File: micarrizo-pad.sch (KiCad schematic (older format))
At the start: 17 parts

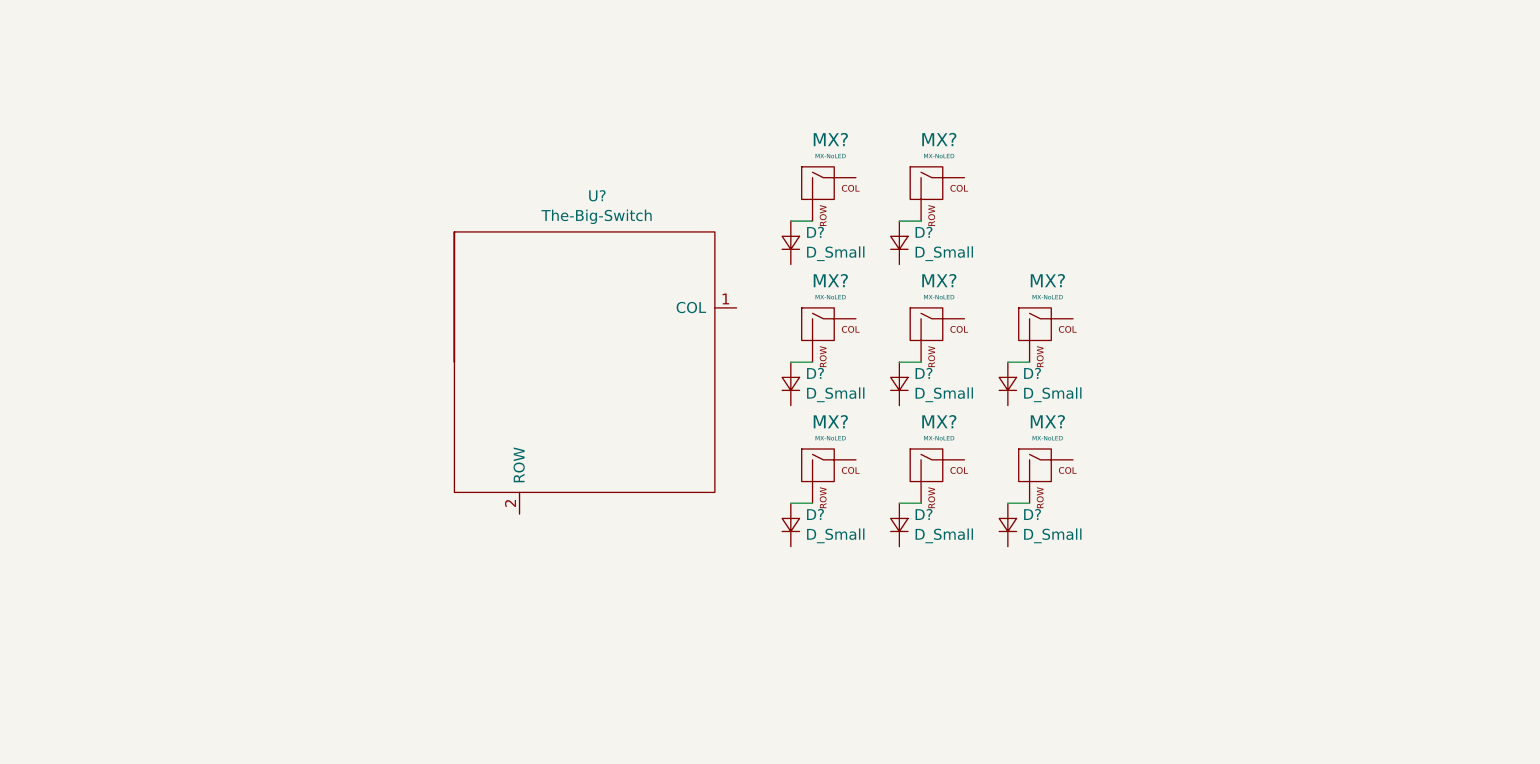
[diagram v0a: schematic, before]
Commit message: add rows cols
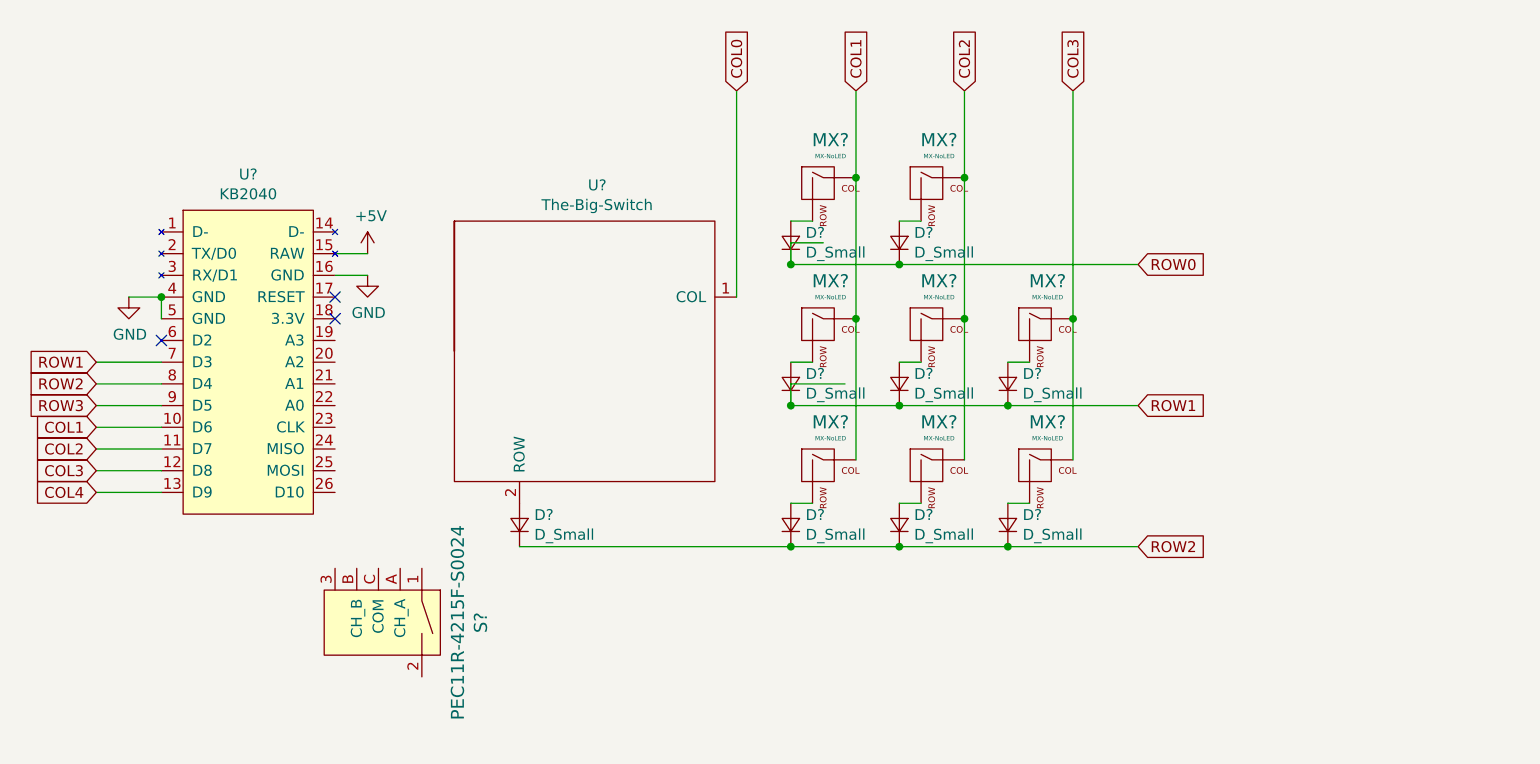
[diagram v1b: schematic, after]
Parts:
- added D?: D_Small, symbol Device:D_Small
- added S?: PEC11R-4215F-S0024, digikey-footprints:Rotary_Encoder_Switched_PEC11R, symbol dk_Encoders:PEC11R-4215F-S0024
- added U?: KB2040, symbol New_Library:KB2040
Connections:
- net labels added: +5V, COL0, COL1, COL2, COL3, COL4, GND, ROW0, ROW1, ROW2, ROW3
- wire segments 8 -> 41
- no-connect marks 0 -> 3
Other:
- moved on the sheet: U?
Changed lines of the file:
@@
 	5750 4300 5850 4300
+$Comp
+L Device:D_Small D?
+U 1 1 65EF06FC
+P 6250 4400
+F 0 "D?" V 6296 4332 50  0000 R CNN
+F 1 "D_Small" V 6205 4332 50  0000 R CNN
+F 2 "" V 6250 4400 50  0001 C CNN
+F 3 "~" V 6250 4400 50  0001 C CNN
+	1    6250 4400
+	0    -1   -1   0
+$EndComp
+Wire Wire Line
+	6250 4300 6350 4300
+$Comp
+L MX_Alps_Hybrid:MX-NoLED MX?
+U 1 1 65EF11E9
+P 6900 4150
+F 0 "MX?" H 6933 4373 60  0000 C CNN
+F 1 "MX-NoLED" H 6933 4299 20  0000 C CNN
+F 2 "" H 6275 4125 60  0001 C CNN
+F 3 "" H 6275 4125 60  0001 C CNN
+	1    6900 4150
+	1    0    0    -1
+$EndComp
+$Comp
+L Device:D_Small D?
+U 1 1 65EF11EF
+P 6750 4400
+F 0 "D?" V 6796 4332 50  0000 R CNN
+F 1 "D_Small" V 6705 4332 50  0000 R CNN
+F 2 "" V 6750 4400 50  0001 C CNN
+F 3 "~" V 6750 4400 50  0001 C CNN
+	1    6750 4400
+	0    -1   -1   0
+$EndComp
+Wire Wire Line
+	6750 4300 6850 4300
+$Comp
+L MX_Alps_Hybrid:MX-NoLED MX?
+U 1 1 65F09C65
+P 5900 2850
+F 0 "MX?" H 5933 3073 60  0000 C CNN
+F 1 "MX-NoLED" H 5933 2999 20  0000 C CNN
+F 2 "" H 5275 2825 60  0001 C CNN
+F 3 "" H 5275 2825 60  0001 C CNN
+	1    5900 2850
+	1    0    0    -1
+$EndComp
+$Comp
+L Device:D_Small D?
+U 1 1 65F09C6B
+P 5750 3100
+F 0 "D?" V 5796 3032 50  0000 R CNN
+F 1 "D_Small" V 5705 3032 50  0000 R CNN
+F 2 "" V 5750 3100 50  0001 C CNN
+F 3 "~" V 5750 3100 50  0001 C CNN
+	1    5750 3100
+	0    -1   -1   0
+$EndComp
+Wire Wire Line
+	5750 3000 5850 3000
+$Comp
+L MX_Alps_Hybrid:MX-NoLED MX?
+U 1 1 65F09C72
+P 6400 2850
+F 0 "MX?" H 6433 3073 60  0000 C CNN
+F 1 "MX-NoLED" H 6433 2999 20  0000 C CNN
+F 2 "" H 5775 2825 60  0001 C CNN
+F 3 "" H 5775 2825 60  0001 C CNN
+	1    6400 2850
+	1    0    0    -1
+$EndComp
+$Comp
+L Device:D_Small D?
+U 1 1 65F09C78
+P 6250 3100
+F 0 "D?" V 6296 3032 50  0000 R CNN
+F 1 "D_Small" V 6205 3032 50  0000 R CNN
+F 2 "" V 6250 3100 50  0001 C CNN
+F 3 "~" V 6250 3100 50  0001 C CNN
+	1    6250 3100
+	0    -1   -1   0
+$EndComp
+Wire Wire Line
+	6250 3000 6350 3000
+$Comp
+L New_Library:The-Big-Switch U?
+U 1 1 65F2656C
+P 4800 3600
+F 0 "U?" H 4858 4365 50  0000 C CNN
+F 1 "The-Big-Switch" H 4858 4274 50  0000 C CNN
+F 2 "" H 4250 4250 50  0001 C CNN
+F 3 "" H 4250 4250 50  0001 C CNN
+	1    4800 3600
+	1    0    0    -1
+$EndComp
+$Comp
+L New_Library:KB2040 U?
+U 1 1 65F497B3
+P 3250 3650
+F 0 "U?" H 3250 4515 50  0000 C CNN
+F 1 "KB2040" H 3250 4424 50  0000 C CNN
+F 2 "" H 3400 4400 50  0001 C CNN
+F 3 "" H 3400 4400 50  0001 C CNN
+	1    3250 3650
+	1    0    0    -1
+$EndComp
+$Comp
+L Device:D_Small D?
+U 1 1 65F4CF1E
+P 4500 4400
+F 0 "D?" V 4546 4332 50  0000 R CNN
+F 1 "D_Small" V 4455 4332 50  0000 R CNN
+F 2 "" V 4500 4400 50  0001 C CNN
+F 3 "~" V 4500 4400 50  0001 C CNN
+	1    4500 4400
+	0    -1   -1   0
+$EndComp
+Wire Wire Line
+	2850 3350 2850 3450
+Wire Wire Line
+	2700 3350 2850 3350
+Connection ~ 2850 3350
+$Comp
+L power:GND #PWR?
+U 1 1 65F4F1ED
+P 2700 3350
+F 0 "#PWR?" H 2700 3100 50  0001 C CNN
+F 1 "GND" H 2705 3177 50  0000 C CNN
+F 2 "" H 2700 3350 50  0001 C CNN
+F 3 "" H 2700 3350 50  0001 C CNN
+	1    2700 3350
+	1    0    0    -1
+$EndComp
+Wire Wire Line
+	3650 3250 3800 3250
+$Comp
+L power:GND #PWR?
+U 1 1 65F51406
+P 3800 3250
+F 0 "#PWR?" H 3800 3000 50  0001 C CNN
+F 1 "GND" H 3805 3077 50  0000 C CNN
+F 2 "" H 3800 3250 50  0001 C CNN
+F 3 "" H 3800 3250 50  0001 C CNN
+	1    3800 3250
+	1    0    0    -1
+$EndComp
+Wire Wire Line
+	3650 3150 3800 3150
+$Comp
+L power:+5V #PWR?
+U 1 1 65F51F24
+P 3800 3150
+F 0 "#PWR?" H 3800 3000 50  0001 C CNN
+F 1 "+5V" H 3815 3323 50  0000 C CNN
+F 2 "" H 3800 3150 50  0001 C CNN
+F 3 "" H 3800 3150 50  0001 C CNN
+	1    3800 3150
+	1    0    0    -1
+$EndComp
+Wire Wire Line
+	4500 4500 5750 4500
+Connection ~ 5750 4500
+Wire Wire Line
+	5750 4500 6250 4500
+Connection ~ 6250 4500
+Wire Wire Line
+	6250 4500 6750 4500
+Connection ~ 6750 4500
+Wire Wire Line
+	6750 4500 7350 4500
+Text GLabel 7350 3850 2    50   Input ~ 0
+ROW1
+Wire Wire Line
+	6000 3750 5750 3750
+Wire Wire Line
+	5750 3750 5750 3850
+Wire Wire Line
+	5750 3850 6250 3850
+Connection ~ 5750 3850
+Connection ~ 6250 3850
+Wire Wire Line
+	6250 3850 6750 3850
+Connection ~ 6750 3850
+Wire Wire Line
+	6750 3850 7350 3850
+Text GLabel 7350 4500 2    50   Input ~ 0
+ROW2
+Wire Wire Line
+	5900 3100 5750 3100
+Wire Wire Line
+	5750 3100 5750 3200
+Wire Wire Line
+	5750 3200 6250 3200
+Connection ~ 5750 3200
+Connection ~ 6250 3200
+Wire Wire Line
+	6250 3200 7350 3200
+Text GLabel 7350 3200 2    50   Input ~ 0
+ROW0
+Wire Wire Line
+	5500 3350 5500 2400
+Text GLabel 6050 2400 1    50   Input ~ 0
+COL1
+Wire Wire Line
+	6050 4100 6050 3450
+Connection ~ 6050 2800
+Wire Wire Line
+	6050 2800 6050 2400
+Connection ~ 6050 3450
+Wire Wire Line
+	6050 3450 6050 2800
+Text GLabel 6550 2400 1    50   Input ~ 0
+COL2
 $Comp
 L MX_Alps_Hybrid:MX-NoLED MX?
@@
 	1    0    0    -1
 $EndComp
-$Comp
-L Device:D_Small D?
-U 1 1 65EF06FC
-P 6250 4400
-F 0 "D?" V 6296 4332 50  0000 R CNN
-F 1 "D_Small" V 6205 4332 50  0000 R CNN
-F 2 "" V 6250 4400 50  0001 C CNN
-F 3 "~" V 6250 4400 50  0001 C CNN
-	1    6250 4400
-	0    -1   -1   0
-$EndComp
-Wire Wire Line
-	6250 4300 6350 4300
-$Comp
-L MX_Alps_Hybrid:MX-NoLED MX?
-U 1 1 65EF11E9
-P 6900 4150
-F 0 "MX?" H 6933 4373 60  0000 C CNN
-F 1 "MX-NoLED" H 6933 4299 20  0000 C CNN
-F 2 "" H 6275 4125 60  0001 C CNN
-F 3 "" H 6275 4125 60  0001 C CNN
-	1    6900 4150
-	1    0    0    -1
-$EndComp
-$Comp
-L Device:D_Small D?
-U 1 1 65EF11EF
-P 6750 4400
-F 0 "D?" V 6796 4332 50  0000 R CNN
-F 1 "D_Small" V 6705 4332 50  0000 R CNN
-F 2 "" V 6750 4400 50  0001 C CNN
-F 3 "~" V 6750 4400 50  0001 C CNN
-	1    6750 4400
-	0    -1   -1   0
-$EndComp
-Wire Wire Line
-	6750 4300 6850 4300
-$Comp
-L MX_Alps_Hybrid:MX-NoLED MX?
-U 1 1 65F09C65
-P 5900 2850
-F 0 "MX?" H 5933 3073 60  0000 C CNN
-F 1 "MX-NoLED" H 5933 2999 20  0000 C CNN
-F 2 "" H 5275 2825 60  0001 C CNN
-F 3 "" H 5275 2825 60  0001 C CNN
-	1    5900 2850
-	1    0    0    -1
-$EndComp
-$Comp
-L Device:D_Small D?
-U 1 1 65F09C6B
-P 5750 3100
-F 0 "D?" V 5796 3032 50  0000 R CNN
-F 1 "D_Small" V 5705 3032 50  0000 R CNN
-F 2 "" V 5750 3100 50  0001 C CNN
-F 3 "~" V 5750 3100 50  0001 C CNN
-	1    5750 3100
-	0    -1   -1   0
-$EndComp
-Wire Wire Line
-	5750 3000 5850 3000
-$Comp
-L MX_Alps_Hybrid:MX-NoLED MX?
-U 1 1 65F09C72
-P 6400 2850
-F 0 "MX?" H 6433 3073 60  0000 C CNN
-F 1 "MX-NoLED" H 6433 2999 20  0000 C CNN
-F 2 "" H 5775 2825 60  0001 C CNN
-F 3 "" H 5775 2825 60  0001 C CNN
-	1    6400 2850
-	1    0    0    -1
-$EndComp
-$Comp
-L Device:D_Small D?
-U 1 1 65F09C78
-P 6250 3100
-F 0 "D?" V 6296 3032 50  0000 R CNN
-F 1 "D_Small" V 6205 3032 50  0000 R CNN
-F 2 "" V 6250 3100 50  0001 C CNN
-F 3 "~" V 6250 3100 50  0001 C CNN
-	1    6250 3100
-	0    -1   -1   0
-$EndComp
-Wire Wire Line
-	6250 3000 6350 3000
-$Comp
-L New_Library:The-Big-Switch U?
-U 1 1 65F2656C
-P 4800 3650
-F 0 "U?" H 4858 4415 50  0000 C CNN
-F 1 "The-Big-Switch" H 4858 4324 50  0000 C CNN
-F 2 "" H 4250 4300 50  0001 C CNN
-F 3 "" H 4250 4300 50  0001 C CNN
-	1    4800 3650
-	1    0    0    -1
+Wire Wire Line
+	6550 2400 6550 2800
+Connection ~ 6550 2800
+Wire Wire Line
+	6550 2800 6550 3450
+Connection ~ 6550 3450
+Wire Wire Line
+	6550 3450 6550 4100
+Text GLabel 7050 2400 1    50   Input ~ 0
+COL3
+Wire Wire Line
+	7050 4100 7050 3450
+Connection ~ 7050 3450
+Wire Wire Line
+	7050 3450 7050 2400
+Text GLabel 5500 2400 1    50   Input ~ 0
+COL0
+Text GLabel 2550 3650 0    50   Input ~ 0
+ROW1
+Text GLabel 2550 3750 0    50   Input ~ 0
+ROW2
+Text GLabel 2550 3850 0    50   Input ~ 0
+ROW3
+Text GLabel 2550 3950 0    50   Input ~ 0
+COL1
+Text GLabel 2550 4050 0    50   Input ~ 0
+COL2
+Text GLabel 2550 4150 0    50   Input ~ 0
+COL3
+Text GLabel 2550 4250 0    50   Input ~ 0
+COL4
+Wire Wire Line
+	2550 3650 2850 3650
+Wire Wire Line
+	2550 3750 2850 3750
+Wire Wire Line
+	2550 3850 2850 3850
+Wire Wire Line
+	2550 3950 2850 3950
+Wire Wire Line
+	2550 4050 2850 4050
+Wire Wire Line
+	2550 4150 2850 4150
+Wire Wire Line
+	2550 4250 2850 4250
+NoConn ~ 2850 3550
+NoConn ~ 3650 3350
+NoConn ~ 3650 3450
+$Comp
+L dk_Encoders:PEC11R-4215F-S0024 S?
+U 1 1 65F65306
+P 3950 4900
+F 0 "S?" H 3900 5272 60  0000 C CNN
+F 1 "PEC11R-4215F-S0024" H 3900 5166 60  0000 C CNN
+F 2 "digikey-footprints:Rotary_Encoder_Switched_PEC11R" H 4150 5100 60  0001 L CNN
+F 3 "https://www.bourns.com/docs/Product-Datasheets/PEC11R.pdf" H 4150 5200 60  0001 L CNN
+F 4 "PEC11R-4215F-S0024-ND" H 4150 5300 60  0001 L CNN "Digi-Key_PN"
+F 5 "PEC11R-4215F-S0024" H 4150 5400 60  0001 L CNN "MPN"
+F 6 "Sensors, Transducers" H 4150 5500 60  0001 L CNN "Category"
+F 7 "Encoders" H 4150 5600 60  0001 L CNN "Family"
+F 8 "https://www.bourns.com/docs/Product-Datasheets/PEC11R.pdf" H 4150 5700 60  0001 L CNN "DK_Datasheet_Link"
+F 9 "/product-detail/en/bourns-inc/PEC11R-4215F-S0024/PEC11R-4215F-S0024-ND/4499665" H 4150 5800 60  0001 L CNN "DK_Detail_Page"
+F 10 "ROTARY ENCODER MECHANICAL 24PPR" H 4150 5900 60  0001 L CNN "Description"
+F 11 "Bourns Inc." H 4150 6000 60  0001 L CNN "Manufacturer"
+F 12 "Active" H 4150 6100 60  0001 L CNN "Status"
+	1    3950 4900
+	0    1    1    0
 $EndComp
 $EndSCHEMATC

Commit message: wire encoder
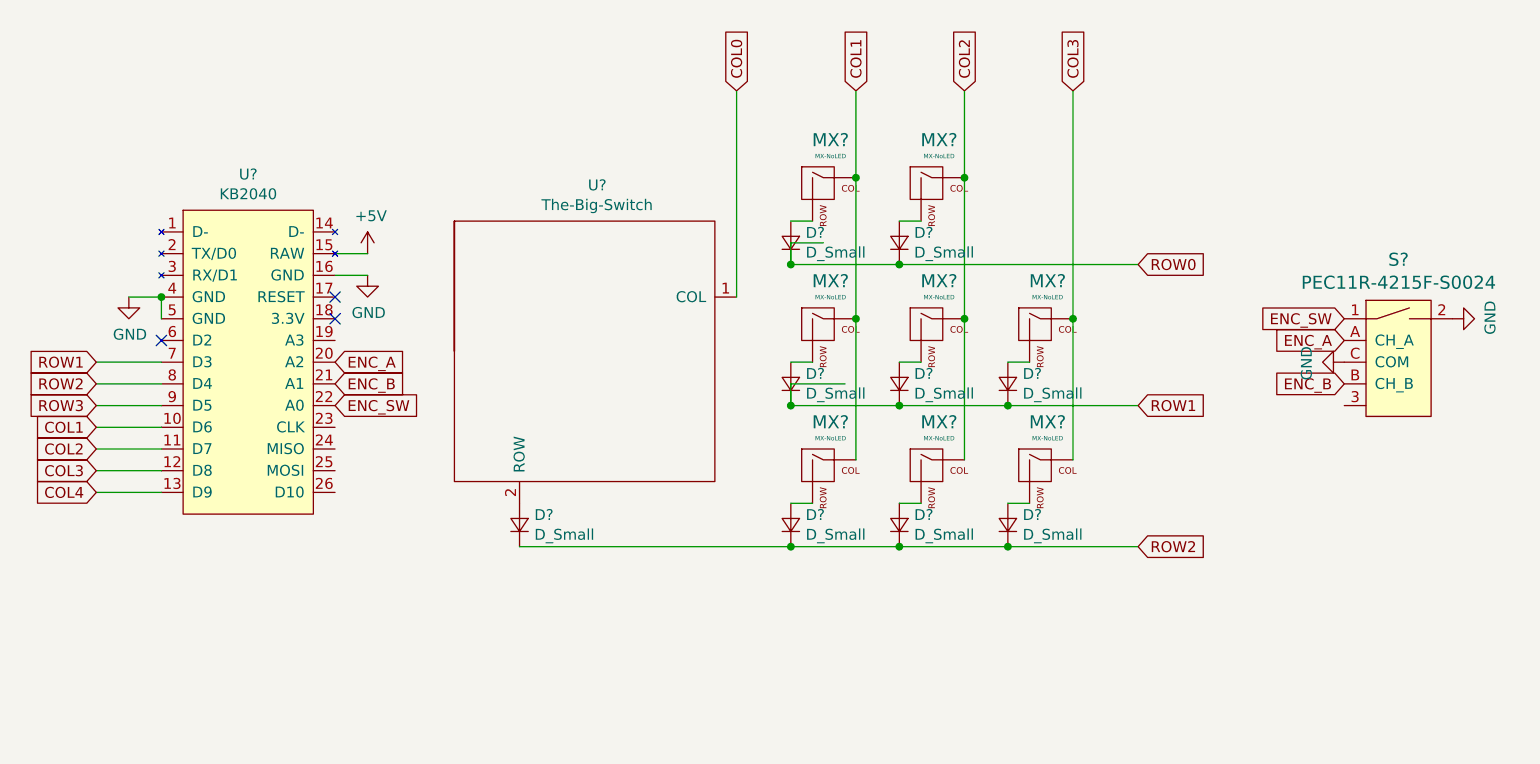
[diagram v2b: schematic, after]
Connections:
- net labels added: ENC_A, ENC_B, ENC_SW
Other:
- moved on the sheet: S?
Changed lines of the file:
@@
 L dk_Encoders:PEC11R-4215F-S0024 S?
 U 1 1 65F65306
-P 3950 4900
-F 0 "S?" H 3900 5272 60  0000 C CNN
-F 1 "PEC11R-4215F-S0024" H 3900 5166 60  0000 C CNN
-F 2 "digikey-footprints:Rotary_Encoder_Switched_PEC11R" H 4150 5100 60  0001 L CNN
-F 3 "https://www.bourns.com/docs/Product-Datasheets/PEC11R.pdf" H 4150 5200 60  0001 L CNN
-F 4 "PEC11R-4215F-S0024-ND" H 4150 5300 60  0001 L CNN "Digi-Key_PN"
-F 5 "PEC11R-4215F-S0024" H 4150 5400 60  0001 L CNN "MPN"
-F 6 "Sensors, Transducers" H 4150 5500 60  0001 L CNN "Category"
-F 7 "Encoders" H 4150 5600 60  0001 L CNN "Family"
-F 8 "https://www.bourns.com/docs/Product-Datasheets/PEC11R.pdf" H 4150 5700 60  0001 L CNN "DK_Datasheet_Link"
-F 9 "/product-detail/en/bourns-inc/PEC11R-4215F-S0024/PEC11R-4215F-S0024-ND/4499665" H 4150 5800 60  0001 L CNN "DK_Detail_Page"
-F 10 "ROTARY ENCODER MECHANICAL 24PPR" H 4150 5900 60  0001 L CNN "Description"
-F 11 "Bourns Inc." H 4150 6000 60  0001 L CNN "Manufacturer"
-F 12 "Active" H 4150 6100 60  0001 L CNN "Status"
-	1    3950 4900
+P 8600 3550
+F 0 "S?" H 8550 3922 60  0000 C CNN
+F 1 "PEC11R-4215F-S0024" H 8550 3816 60  0000 C CNN
+F 2 "digikey-footprints:Rotary_Encoder_Switched_PEC11R" H 8800 3750 60  0001 L CNN
+F 3 "https://www.bourns.com/docs/Product-Datasheets/PEC11R.pdf" H 8800 3850 60  0001 L CNN
+F 4 "PEC11R-4215F-S0024-ND" H 8800 3950 60  0001 L CNN "Digi-Key_PN"
+F 5 "PEC11R-4215F-S0024" H 8800 4050 60  0001 L CNN "MPN"
+F 6 "Sensors, Transducers" H 8800 4150 60  0001 L CNN "Category"
+F 7 "Encoders" H 8800 4250 60  0001 L CNN "Family"
+F 8 "https://www.bourns.com/docs/Product-Datasheets/PEC11R.pdf" H 8800 4350 60  0001 L CNN "DK_Datasheet_Link"
+F 9 "/product-detail/en/bourns-inc/PEC11R-4215F-S0024/PEC11R-4215F-S0024-ND/4499665" H 8800 4450 60  0001 L CNN "DK_Detail_Page"
+F 10 "ROTARY ENCODER MECHANICAL 24PPR" H 8800 4550 60  0001 L CNN "Description"
+F 11 "Bourns Inc." H 8800 4650 60  0001 L CNN "Manufacturer"
+F 12 "Active" H 8800 4750 60  0001 L CNN "Status"
+	1    8600 3550
+	1    0    0    -1
+$EndComp
+$Comp
+L power:GND #PWR?
+U 1 1 65FB7F76
+P 8800 3450
+F 0 "#PWR?" H 8800 3200 50  0001 C CNN
+F 1 "GND" H 8805 3277 50  0000 C CNN
+F 2 "" H 8800 3450 50  0001 C CNN
+F 3 "" H 8800 3450 50  0001 C CNN
+	1    8800 3450
+	0    -1   -1   0
+$EndComp
+$Comp
+L power:GND #PWR?
+U 1 1 65FB99F0
+P 8300 3650
+F 0 "#PWR?" H 8300 3400 50  0001 C CNN
+F 1 "GND" H 8305 3477 50  0000 C CNN
+F 2 "" H 8300 3650 50  0001 C CNN
+F 3 "" H 8300 3650 50  0001 C CNN
+	1    8300 3650
 	0    1    1    0
 $EndComp
+Text GLabel 8300 3450 0    50   Input ~ 0
+ENC_SW
+Text GLabel 8300 3550 0    50   Input ~ 0
+ENC_A
+Text GLabel 8300 3750 0    50   Input ~ 0
+ENC_B
+Text GLabel 3650 3850 2    50   Input ~ 0
+ENC_SW
+Text GLabel 3650 3650 2    50   Input ~ 0
+ENC_A
+Text GLabel 3650 3750 2    50   Input ~ 0
+ENC_B
 $EndSCHEMATC
